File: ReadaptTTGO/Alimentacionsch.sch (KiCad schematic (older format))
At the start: 12 parts

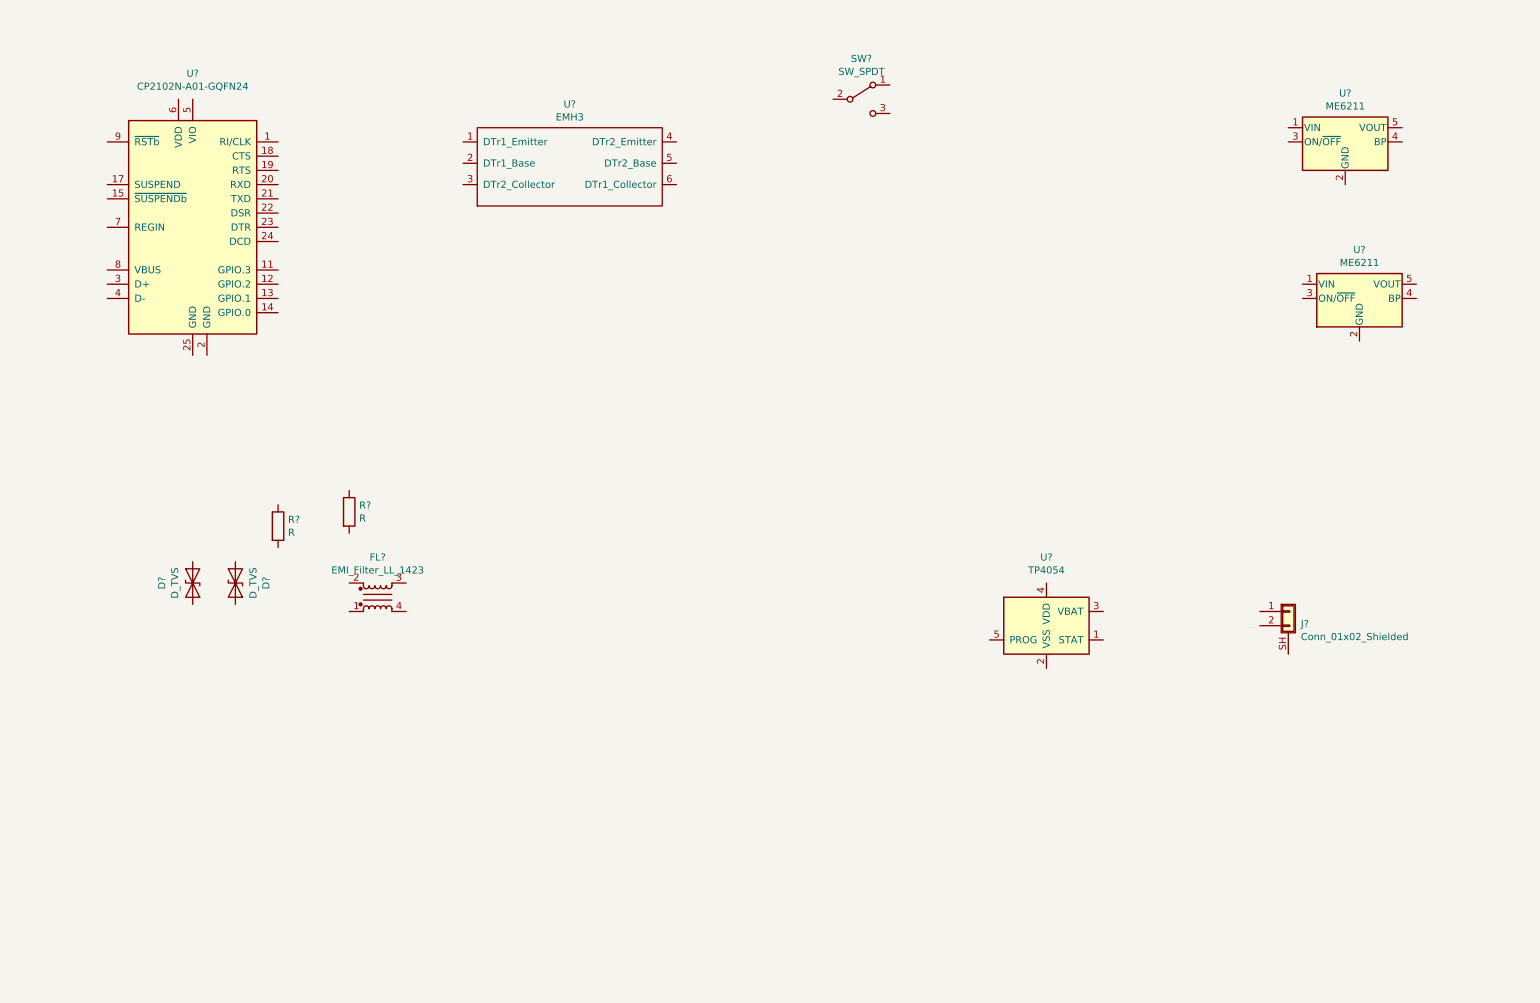
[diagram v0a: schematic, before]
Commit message: Primer aproximacion.
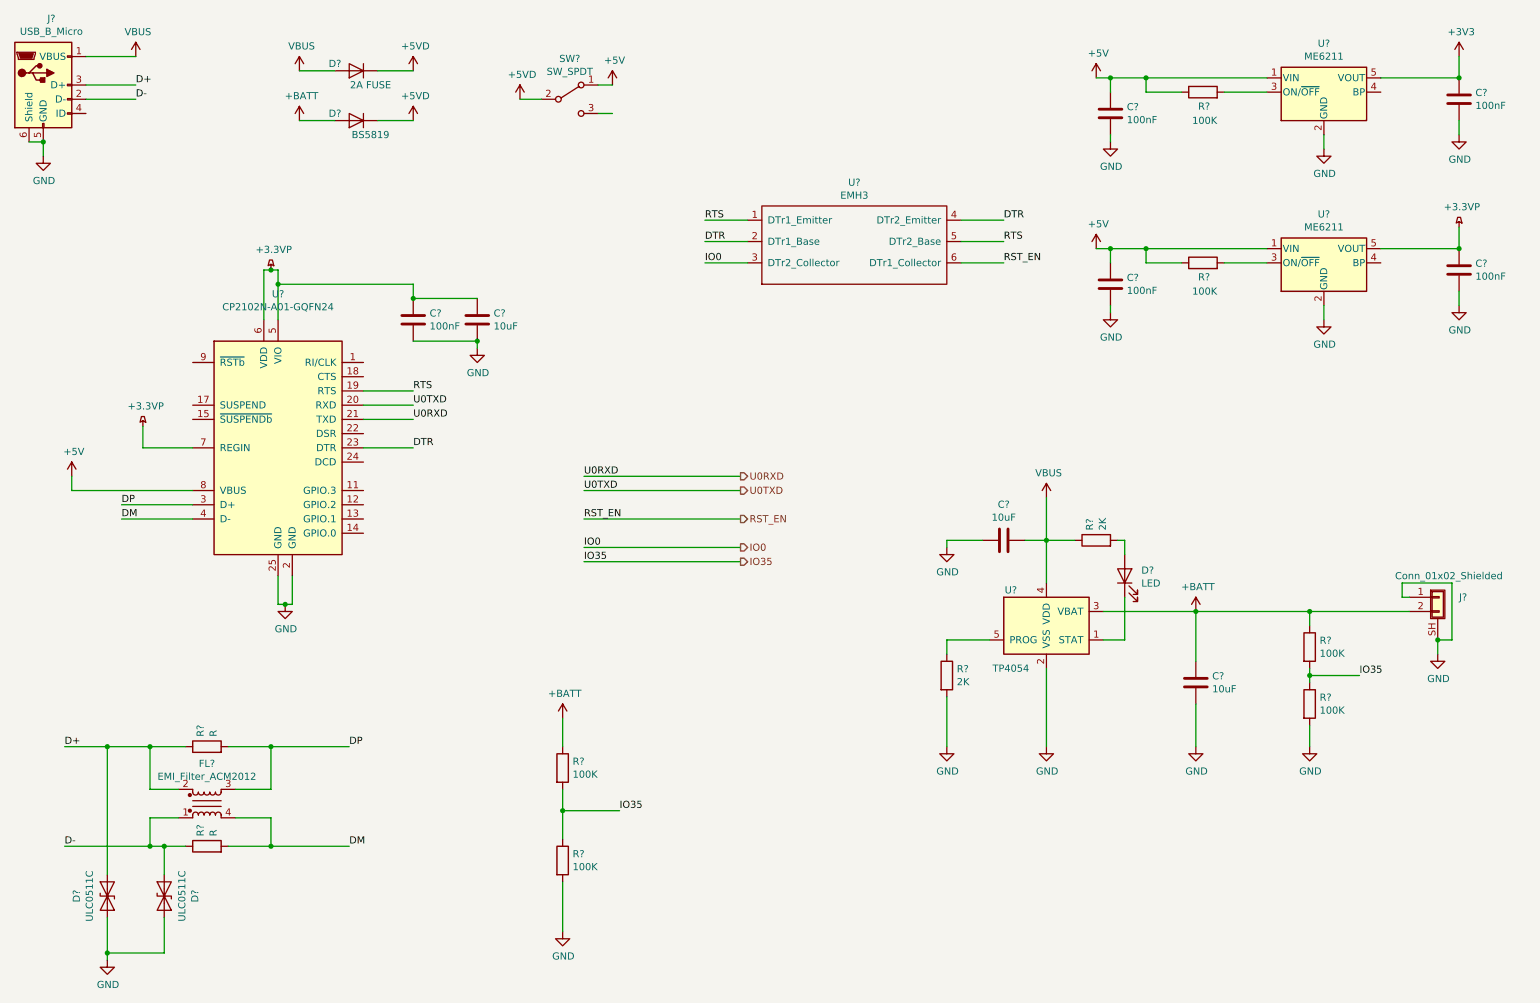
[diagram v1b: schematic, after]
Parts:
- added C? (x5): 100nF, symbol Device:C
- added C? (x3): 10uF, symbol Device:C
- added D?: LED, symbol Device:LED
- added D?: 2A FUSE, symbol Device:D
- added D?: BS5819, symbol Device:D
- added J?: USB_B_Micro, symbol Connector:USB_B_Micro
- added R? (x6): 100K, symbol Device:R
- added R? (x2): 2K, symbol Device:R
- D? (x2): value D_TVS -> ULC0511C
- FL?: value EMI_Filter_LL_1423 -> EMI_Filter_ACM2012
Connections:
- net at U?.1 (STAT): now also D?.1 (K)
- net GND: now reaches U?.2 (VSS)
- net GND: now also D?.1 (A1), D?.2 (A2), J?.1 (Pin_1), J?.SH (Shield), U?.2 (GND), U?.2 (GND), U?.2 (GND), U?.25 (GND), C?.2, C?.2, C?.2, C?.2, C?.2, C?.2, C?.2, C?.2, J?.5 (GND), J?.6 (Shield), R?.2, R?.2, R?.2
- net +BATT: now reaches U?.3 (VBAT)
- net +BATT: now also J?.2 (Pin_2), C?.1, D?.2 (A), R?.1, R?.1
- net VBUS: now reaches U?.4 (VDD)
- net VBUS: now also C?.1, D?.2 (A), J?.1 (VBUS), R?.1
- net at U?.5 (PROG): now also R?.1
- net RTS: now reaches U?.19 (RTS)
- net RTS: now also U?.1 (DTr1_Emitter), U?.5 (DTr2_Base)
- net U0TXD: now reaches U?.20 (RXD)
- net U0RXD: now reaches U?.21 (TXD)
- net DTR: now reaches U?.23 (DTR)
- net DTR: now also U?.2 (DTr1_Base), U?.4 (DTr2_Emitter)
- net DP: now reaches U?.3 (D+)
- net DP: now also FL?.3, R?.2
- net DM: now reaches U?.4 (D-)
- net DM: now also FL?.4, R?.2
- net +3.3VP: now reaches U?.5 (VIO)
- net +3.3VP: now also U?.5 (VOUT), U?.6 (VDD), U?.7 (REGIN), C?.1, C?.1, C?.1
- net +5V: now reaches U?.8 (VBUS)
- net +5V: now also SW?.1 (A), U?.1 (VIN), U?.1 (VIN), C?.1, C?.1, R?.1, R?.1
- net IO0: now reaches U?.3 (DTr2_Collector)
- net RST_EN: now reaches U?.6 (DTr1_Collector)
- net at U?.3 (ON/~OFF~): now also R?.2 (x2)
- net +3V3: now reaches U?.5 (VOUT)
- net +3V3: now also C?.1
- net D-: now reaches FL?.1
- net D-: now also D?.1 (A1), R?.1, J?.2 (D-)
- net D+: now reaches FL?.2
- net D+: now also D?.2 (A2), R?.1, J?.3 (D+)
- net +5VD: now reaches SW?.2 (B)
- net +5VD: now also D?.1 (K), D?.1 (K)
- new net: D?.2 (A), R?.2
- new net IO35: R?.1, R?.1, R?.2, R?.2
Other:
- moved on the sheet: D?, FL?, J?, R?, SW?, U?
